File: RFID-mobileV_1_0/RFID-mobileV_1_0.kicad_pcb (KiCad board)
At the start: 2 copper layers, 50.7 x 89.5 mm, 54 parts, among them J1 USB_C_Receptacle_USB2.0, J2 Conn_01x05_Male, J3 Conn_01x05_Female, J4 Conn_01x05_Male, Q1 MMBT3904, SW1 SW_Push, U1 XC6206P332MR, U2 E22-400T22S, U3 STM32G030FxP, U4 LM321, U5 DW02, U6 TP4054

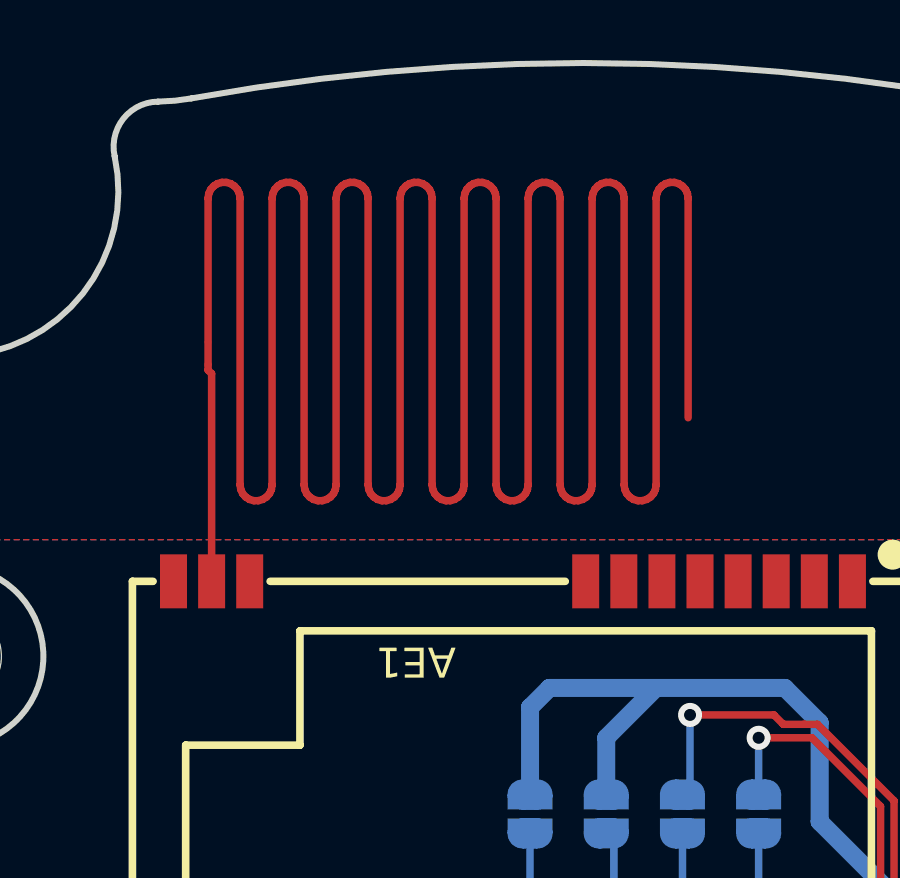
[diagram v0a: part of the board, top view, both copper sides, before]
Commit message: update
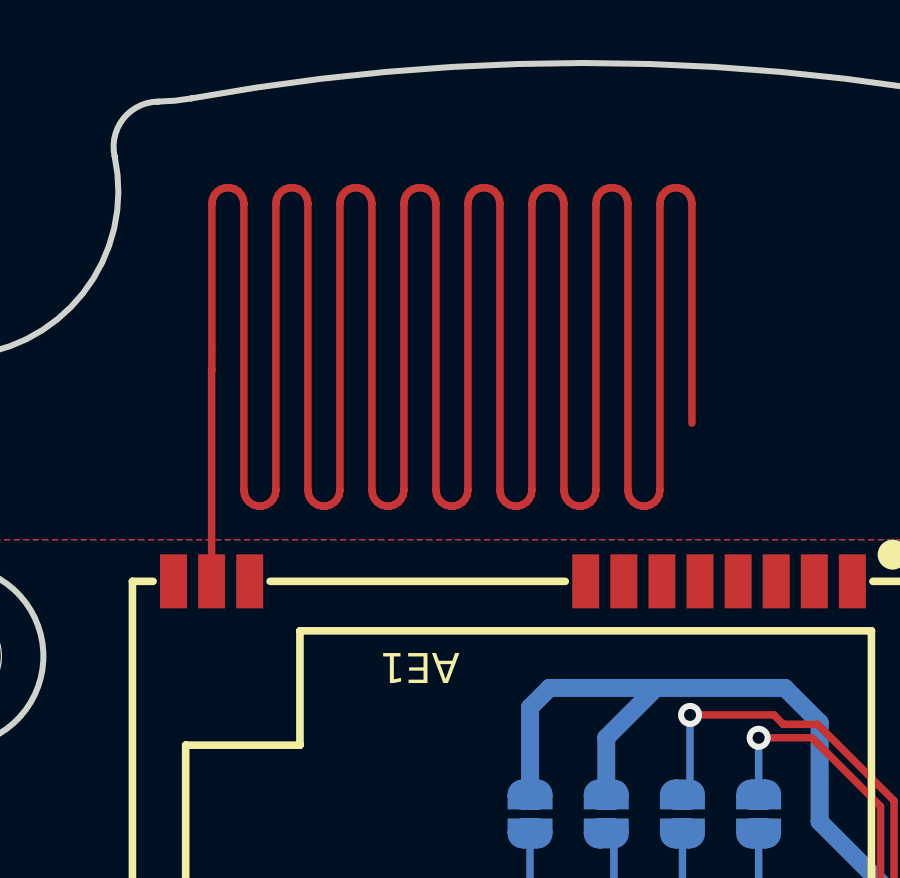
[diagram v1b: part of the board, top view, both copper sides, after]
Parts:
- moved AE1 0.22 mm to (85.0, 90.6)
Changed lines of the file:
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@@
   )
   (footprint "RF_Antenna:433MHz_V" (layer "F.Cu")
-    (at 84.836 90.424 180)
+    (at 84.963 90.6018 180)
     (property "Sheetfile" "RFID-mobileV_1_0.kicad_sch")
     (property "Sheetname" "")
@@
   (gr_arc locked (start 66.16277 161.39279) (mid 64.73449 161.282141) (end 64.050435 160.023467) (layer "Edge.Cuts") (width 0.2))
   (gr_circle locked (center 110.407996 100.913642) (end 113.407996 100.913642) (layer "Edge.Cuts") (width 0.2) (fill none))
-  (segment (start 77.016 91.494) (end 77.016 98.417) (width 0.25) (layer "F.Cu") (net 1))
-  (segment (start 76.8975 91.186) (end 76.8975 91.3755) (width 0.25) (layer "F.Cu") (net 1))
-  (segment (start 76.8975 91.3755) (end 77.016 91.494) (width 0.25) (layer "F.Cu") (net 1))
+  (segment (start 77.016 91.3723) (end 77.016 98.417) (width 0.25) (layer "F.Cu") (net 1))
+  (segment (start 77.0245 91.3638) (end 77.016 91.3723) (width 0.25) (layer "F.Cu") (net 1))
   (segment (start 78.867 158.4995) (end 78.867 160.401) (width 0.6) (layer "F.Cu") (net 2))
   (segment (start 74.102 145.984) (end 76.2 145.984) (width 0.6) (layer "F.Cu") (net 2))
